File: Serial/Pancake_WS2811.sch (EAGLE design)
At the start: 14 parts

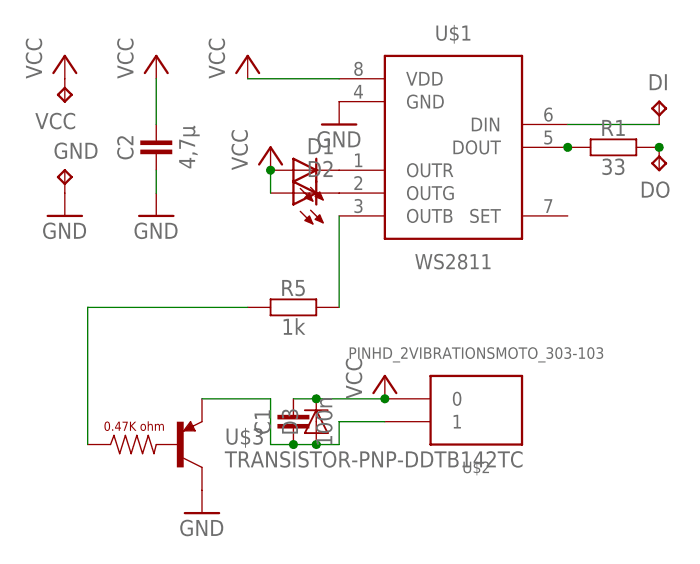
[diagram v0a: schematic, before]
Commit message: Update pictures, pancake
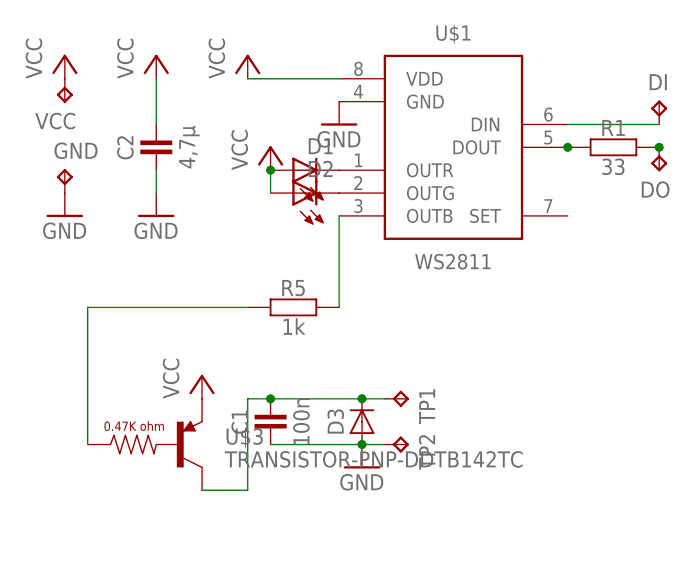
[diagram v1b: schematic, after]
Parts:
- removed U$2: PINHD_2VIBRATIONSMOTO_303-103, thar:PINHD_2VIBRATIONSMOTO_303-103
- added TP1, TP2: TPTP20R, testpad:TPTP20R
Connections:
- removed net N$4: C1.1, D3.A, U$2.1, U$3.E
- new net N$1: C1.2, D3.C, TP1.TP, U$3.C
- net GND: now also C1.1, D3.A, TP2.TP; no longer U$3.C
- net VCC: now also U$3.E; no longer C1.2, D3.C, U$2.0
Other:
- moved on the sheet: C1, D3
